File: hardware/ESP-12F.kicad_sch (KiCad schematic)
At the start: 29 parts, among them U10 ESP-12F, U11 MCP2558FD-xMF, U8 PI4IOE5V6416LEX, U9 PI4IOE5V6416LEX

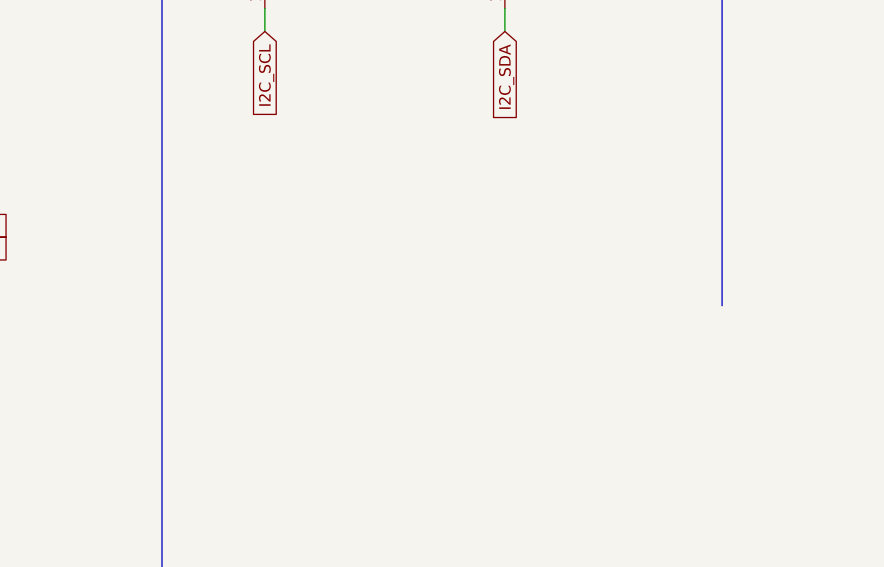
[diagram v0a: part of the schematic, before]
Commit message: working assighning footprints still
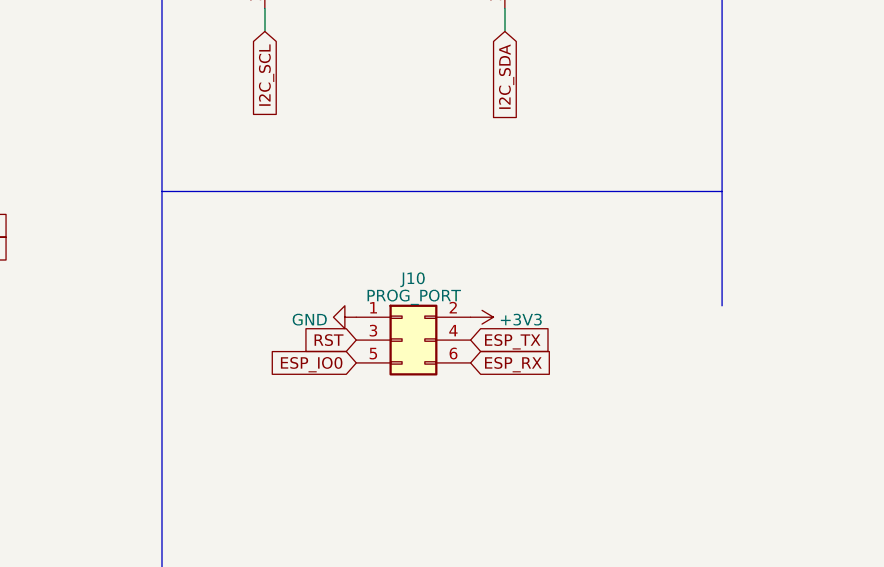
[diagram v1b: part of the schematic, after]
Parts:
- added J10: PROG_PORT, symbol Connector_Generic:Conn_02x03_Odd_Even
- R50, R51, R52, R53, R54, R55, R56, R57, R58, R59, R60, R61: footprint (none) -> Resistor_SMD:R_0603_1608Metric
- U8, U9: footprint (none) -> PCM_Package_SO_AKL:TSSOP-24_4.4x7.8mm_P0.65mm
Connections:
- net +3V3: now also J10.2 (Pin_2)
- net ESP_IO0: now also J10.5 (Pin_5)
- net ESP_RX: now also J10.6 (Pin_6)
- net ESP_TX: now also J10.4 (Pin_4)
- net GND: now also J10.1 (Pin_1)
- net RST: now also J10.3 (Pin_3)
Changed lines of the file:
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@@
+    (stroke (width 0) (type default))
+  )
+  (polyline (pts (xy 115.57 153.67) (xy 177.8 153.67))
     (stroke (width 0) (type default))
   )
@@
     (effects (font (size 1.27 1.27)) (justify left bottom))
   )
+  (global_label "ESP_TX" (shape input) (at 149.86 170.18 0) (fields_autoplaced)
+    (effects (font (size 1.27 1.27)) (justify left))
+    (property "Intersheetrefs" "${INTERSHEET_REFS}" (at 159.539 170.18 0)
+      (effects (font (size 1.27 1.27)) (justify left) hide)
+    )
+  )
   (global_label "B_SUB-C_BUCK_P-GOOD" (shape input) (at 85.09 55.88 0) (fields_autoplaced)
     (effects (font (size 1.27 1.27)) (justify left))
@@
     (property "Intersheetrefs" "${INTERSHEET_REFS}" (at 111.6419 88.9 0)
       (effects (font (size 1.27 1.27)) (justify left) hide)
+    )
+  )
+  (global_label "RST" (shape input) (at 137.16 170.18 180) (fields_autoplaced)
+    (effects (font (size 1.27 1.27)) (justify right))
+    (property "Intersheetrefs" "${INTERSHEET_REFS}" (at 130.8071 170.18 0)
+      (effects (font (size 1.27 1.27)) (justify right) hide)
     )
   )
@@
     )
   )
+  (global_label "ESP_IO0" (shape input) (at 137.16 172.72 180) (fields_autoplaced)
+    (effects (font (size 1.27 1.27)) (justify right))
+    (property "Intersheetrefs" "${INTERSHEET_REFS}" (at 126.5133 172.72 0)
+      (effects (font (size 1.27 1.27)) (justify right) hide)
+    )
+  )
   (global_label "ESP_RX" (shape input) (at 220.98 58.42 0) (fields_autoplaced)
     (effects (font (size 1.27 1.27)) (justify left))
@@
     )
   )
+  (global_label "ESP_RX" (shape input) (at 149.86 172.72 0) (fields_autoplaced)
+    (effects (font (size 1.27 1.27)) (justify left))
+    (property "Intersheetrefs" "${INTERSHEET_REFS}" (at 159.8414 172.72 0)
+      (effects (font (size 1.27 1.27)) (justify left) hide)
+    )
+  )
   (global_label "DFP_C_ATTACH_1" (shape input) (at 85.09 129.54 0) (fields_autoplaced)
     (effects (font (size 1.27 1.27)) (justify left))
@@
       (effects (font (size 1.27 1.27)) (justify left))
     )
-    (property "Footprint" "" (at 36.322 144.78 90)
+    (property "Footprint" "Resistor_SMD:R_0603_1608Metric" (at 36.322 144.78 90)
       (effects (font (size 1.27 1.27)) hide)
     )
@@
       (effects (font (size 1.27 1.27)) (justify left))
     )
-    (property "Footprint" "" (at 146.812 67.31 90)
+    (property "Footprint" "Resistor_SMD:R_0603_1608Metric" (at 146.812 67.31 90)
       (effects (font (size 1.27 1.27)) hide)
     )
@@
       (effects (font (size 1.27 1.27)) (justify left))
     )
-    (property "Footprint" "" (at 217.932 81.28 90)
+    (property "Footprint" "Resistor_SMD:R_0603_1608Metric" (at 217.932 81.28 90)
       (effects (font (size 1.27 1.27)) hide)
     )
@@
       (effects (font (size 1.27 1.27)) (justify left))
     )
-    (property "Footprint" "" (at 36.322 76.2 90)
+    (property "Footprint" "Resistor_SMD:R_0603_1608Metric" (at 36.322 76.2 90)
       (effects (font (size 1.27 1.27)) hide)
     )
@@
       (effects (font (size 1.27 1.27)) (justify left))
     )
-    (property "Footprint" "" (at 254.762 138.43 90)
+    (property "Footprint" "Resistor_SMD:R_0603_1608Metric" (at 254.762 138.43 90)
       (effects (font (size 1.27 1.27)) hide)
     )
@@
       (effects (font (size 1.27 1.27)) (justify left))
     )
-    (property "Footprint" "" (at 263.652 39.37 90)
+    (property "Footprint" "Resistor_SMD:R_0603_1608Metric" (at 263.652 39.37 90)
       (effects (font (size 1.27 1.27)) hide)
     )
@@
     )
   )
+  (symbol (lib_id "power:GND") (at 137.16 167.64 270) (unit 1)
+    (in_bom yes) (on_board yes) (dnp no) (fields_autoplaced)
+    (property "Reference" "#PWR0146" (at 130.81 167.64 0)
+      (effects (font (size 1.27 1.27)) hide)
+    )
+    (property "Value" "GND" (at 133.9851 167.9568 90)
+      (effects (font (size 1.27 1.27)) (justify right))
+    )
+    (property "Footprint" "" (at 137.16 167.64 0)
+      (effects (font (size 1.27 1.27)) hide)
+    )
+    (property "Datasheet" "" (at 137.16 167.64 0)
+      (effects (font (size 1.27 1.27)) hide)
+    )
+    (pin "1")
+    (instances
+      (project "usbc-car-module"
+        (path "/fae025e9-99c5-40c1-af6f-99dc1edbfa43/62352716-6578-44e5-ac45-fc6ae860b12d"
+          (reference "#PWR0146") (unit 1)
+        )
+      )
+    )
+  )
   (symbol (lib_id "Device:C") (at 255.27 39.37 0) (unit 1)
     (in_bom yes) (on_board yes) (dnp no) (fields_autoplaced)
@@
       (effects (font (size 1.27 1.27)) (justify left))
     )
-    (property "Footprint" "" (at 178.562 39.37 90)
+    (property "Footprint" "Resistor_SMD:R_0603_1608Metric" (at 178.562 39.37 90)
       (effects (font (size 1.27 1.27)) hide)
     )
@@
         (path "/fae025e9-99c5-40c1-af6f-99dc1edbfa43/62352716-6578-44e5-ac45-fc6ae860b12d"
           (reference "R55") (unit 1)
+        )
+      )
+    )
+  )
+  (symbol (lib_id "power:+3V3") (at 149.86 167.64 270) (unit 1)
+    (in_bom yes) (on_board yes) (dnp no) (fields_autoplaced)
+    (property "Reference" "#PWR0147" (at 146.05 167.64 0)
+      (effects (font (size 1.27 1.27)) hide)
+    )
+    (property "Value" "+3V3" (at 153.035 167.9568 90)
+      (effects (font (size 1.27 1.27)) (justify left))
+    )
+    (property "Footprint" "" (at 149.86 167.64 0)
+      (effects (font (size 1.27 1.27)) hide)
+    )
+    (property "Datasheet" "" (at 149.86 167.64 0)
+      (effects (font (size 1.27 1.27)) hide)
+    )
+    (pin "1")
+    (instances
+      (project "usbc-car-module"
+        (path "/fae025e9-99c5-40c1-af6f-99dc1edbfa43/62352716-6578-44e5-ac45-fc6ae860b12d"
+          (reference "#PWR0147") (unit 1)
         )
       )
@@
       (effects (font (size 1.27 1.27)) (justify left))
     )
-    (property "Footprint" "" (at 69.85 106.68 0)
+    (property "Footprint" "PCM_Package_SO_AKL:TSSOP-24_4.4x7.8mm_P0.65mm" (at 69.85 106.68 0)
       (effects (font (size 1.27 1.27)) hide)
     )
@@
       (effects (font (size 1.27 1.27)) (justify left))
     )
-    (property "Footprint" "" (at 155.702 39.37 90)
+    (property "Footprint" "Resistor_SMD:R_0603_1608Metric" (at 155.702 39.37 90)
       (effects (font (size 1.27 1.27)) hide)
     )
@@
       (effects (font (size 1.27 1.27)) (justify left))
     )
-    (property "Footprint" "" (at 69.85 38.1 0)
+    (property "Footprint" "PCM_Package_SO_AKL:TSSOP-24_4.4x7.8mm_P0.65mm" (at 69.85 38.1 0)
       (effects (font (size 1.27 1.27)) hide)
     )
@@
       (effects (font (size 1.27 1.27)) (justify left))
     )
-    (property "Footprint" "" (at 219.202 39.37 90)
+    (property "Footprint" "Resistor_SMD:R_0603_1608Metric" (at 219.202 39.37 90)
       (effects (font (size 1.27 1.27)) hide)
     )
@@
       (effects (font (size 1.27 1.27)) (justify left))
     )
-    (property "Footprint" "" (at 271.272 39.37 90)
+    (property "Footprint" "Resistor_SMD:R_0603_1608Metric" (at 271.272 39.37 90)
       (effects (font (size 1.27 1.27)) hide)
     )
@@
     )
   )
+  (symbol (lib_id "Connector_Generic:Conn_02x03_Odd_Even") (at 142.24 170.18 0) (unit 1)
+    (in_bom yes) (on_board yes) (dnp no) (fields_autoplaced)
+    (property "Reference" "J10" (at 143.51 163.3601 0)
+      (effects (font (size 1.27 1.27)))
+    )
+    (property "Value" "PROG_PORT" (at 143.51 165.2811 0)
+      (effects (font (size 1.27 1.27)))
+    )
+    (property "Footprint" "" (at 142.24 170.18 0)
+      (effects (font (size 1.27 1.27)) hide)
+    )
+    (property "Datasheet" "~" (at 142.24 170.18 0)
+      (effects (font (size 1.27 1.27)) hide)
+    )
+    (pin "1")
+    (pin "2")
+    (pin "3")
+    (pin "4")
+    (pin "5")
+    (pin "6")
+    (instances
+      (project "usbc-car-module"
+        (path "/fae025e9-99c5-40c1-af6f-99dc1edbfa43/62352716-6578-44e5-ac45-fc6ae860b12d"
+          (reference "J10") (unit 1)
+        )
+      )
+    )
+  )
   (symbol (lib_id "Device:R") (at 148.59 54.61 0) (unit 1)
     (in_bom yes) (on_board yes) (dnp no) (fields_autoplaced)
@@
       (effects (font (size 1.27 1.27)) (justify left))
     )
-    (property "Footprint" "" (at 146.812 54.61 90)
+    (property "Footprint" "Resistor_SMD:R_0603_1608Metric" (at 146.812 54.61 90)
       (effects (font (size 1.27 1.27)) hide)
     )
@@
       (effects (font (size 1.27 1.27)) (justify left))
     )
-    (property "Footprint" "" (at 225.552 81.28 90)
-      (effects (font (size 1.27 1.27)) hide)
-    )
+    (property "Footprint" "Resistor_SMD:R_0603_1608Metric" (at 225.552 81.28 90)
+      (effects (font (size 1.27 1.27)) hide)
+    )

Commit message: FINALY starting the pcb
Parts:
- J10: footprint (none) -> Connector_PinHeader_2.54mm:PinHeader_2x03_P2.54mm_Vertical
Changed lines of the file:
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@@
       (effects (font (size 1.27 1.27)))
     )
-    (property "Footprint" "" (at 142.24 170.18 0)
+    (property "Footprint" "Connector_PinHeader_2.54mm:PinHeader_2x03_P2.54mm_Vertical" (at 142.24 170.18 0)
       (effects (font (size 1.27 1.27)) hide)
     )
